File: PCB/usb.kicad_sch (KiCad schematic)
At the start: 53 parts, among them J2 Conn_ARM_SWD_TagConnect_TC2030, J4 TYPE-C-31-M-12, U10 FT2232HQ, U3 TPD2EUSB30, U4 TPD2EUSB30, U6 TPD2EUSB30, U8 TPS62132, U9 M93C56-WMN6TP, Y2 12MHz

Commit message: fixing a bunch of footprints to standardize
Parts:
- C124: footprint Capacitor_SMD:C_0402_1005Metric -> Capacitor_SMD:C_0603_1608Metric
- C92: footprint Capacitor_SMD:C_0402_1005Metric -> Capacitor_SMD:C_1206_3216Metric
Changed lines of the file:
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@@
 			)
 		)
-		(property "Footprint" "Capacitor_SMD:C_0402_1005Metric"
+		(property "Footprint" "Capacitor_SMD:C_0603_1608Metric"
 			(at 97.4852 38.1 0)
 			(effects
@@
 			)
 		)
-		(property "Footprint" "Capacitor_SMD:C_0402_1005Metric"
+		(property "Footprint" "Capacitor_SMD:C_1206_3216Metric"
 			(at 195.2752 48.26 0)
 			(effects

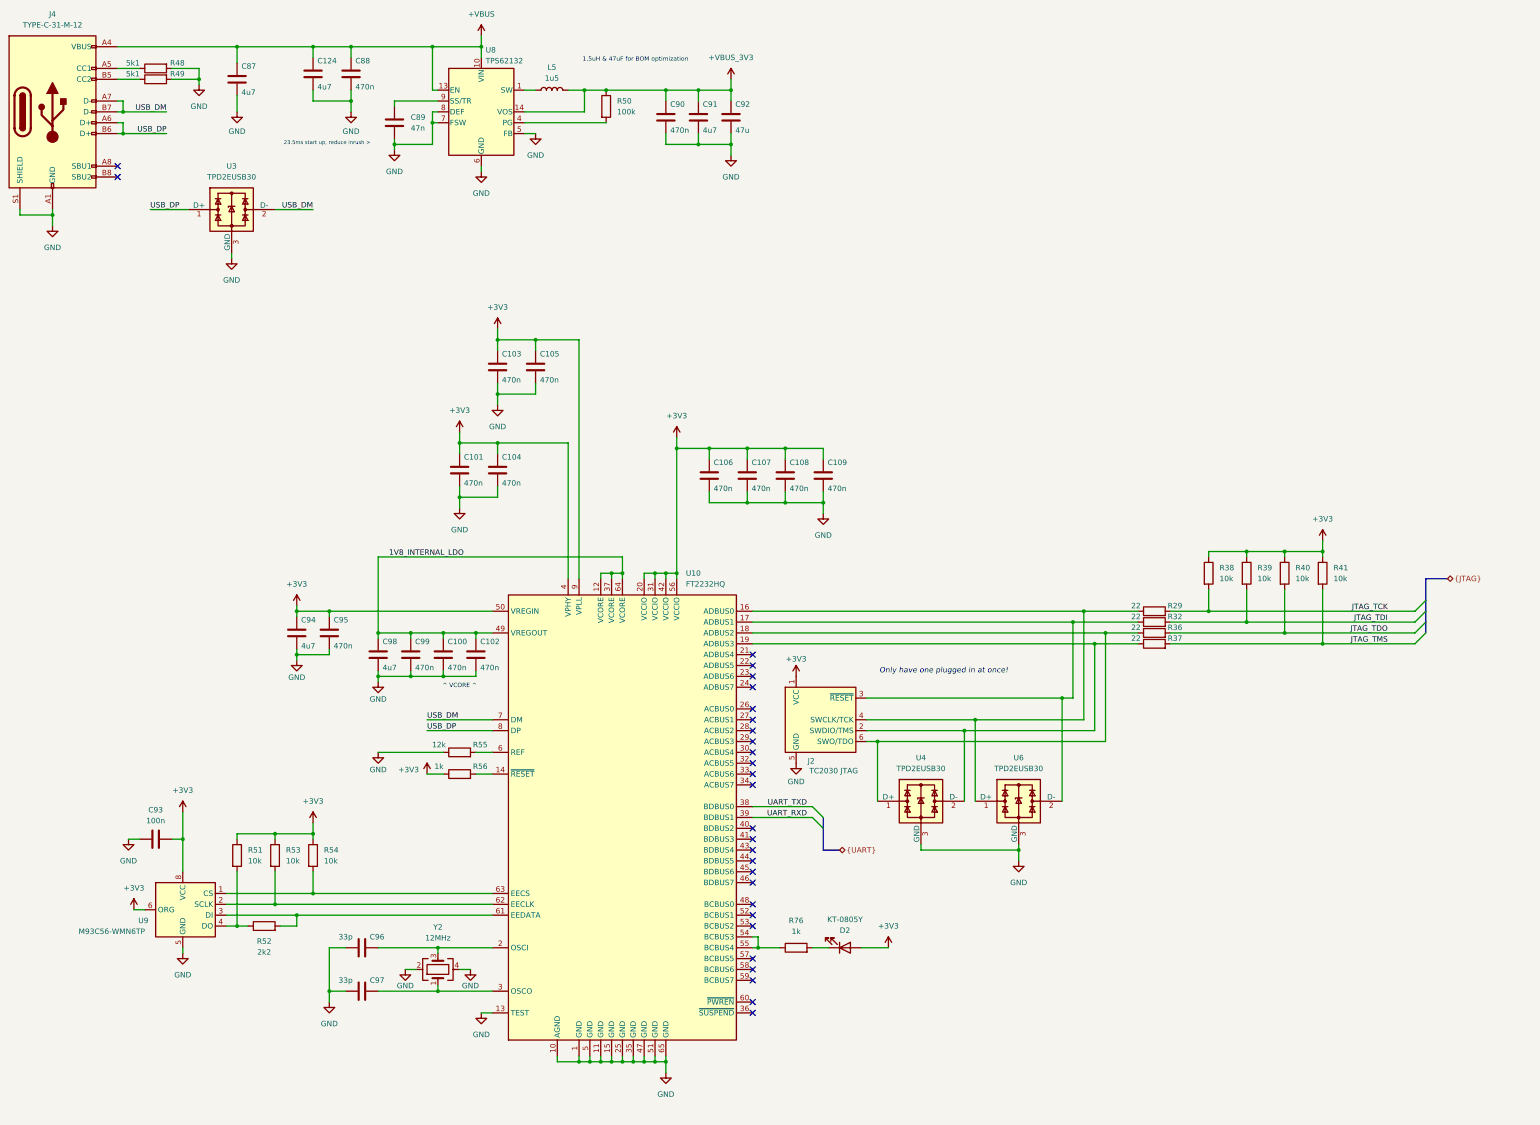
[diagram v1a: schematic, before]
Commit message: workingng on organizing the board
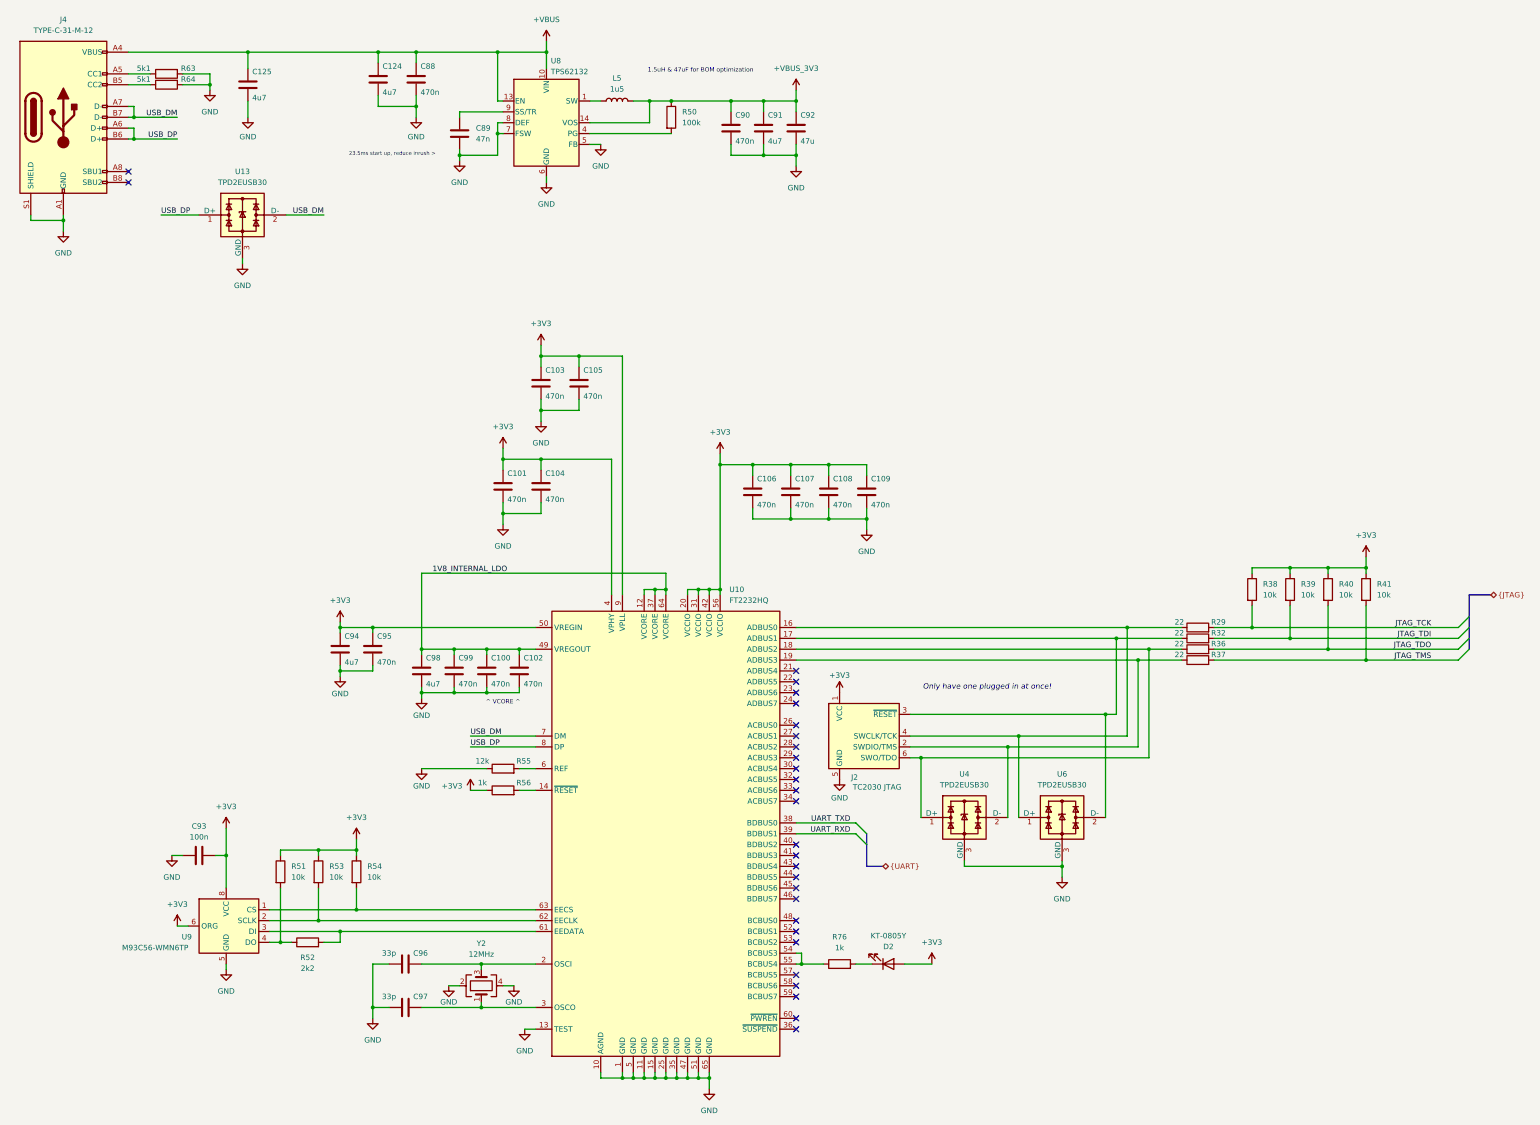
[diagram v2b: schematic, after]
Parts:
- removed C87: 4u7, Capacitor_SMD:C_0603_1608Metric, symbol Device:C
- removed R48, R49: 5k1, Resistor_SMD:R_0402_1005Metric, symbol Device:R
- removed U3: TPD2EUSB30, Package_TO_SOT_SMD:Texas_DRT-3, symbol Power_Protection:TPD2EUSB30
- added C125: 4u7, Capacitor_SMD:C_0603_1608Metric, symbol Device:C
- added R63, R64: 5k1, Resistor_SMD:R_0402_1005Metric, symbol Device:R
- added U13: TPD2EUSB30, Package_TO_SOT_SMD:Texas_DRT-3, symbol Power_Protection:TPD2EUSB30
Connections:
- net +VBUS: now also C125.1
- net GND: now also C125.2, R63.2, R64.2, U13.3 (GND)
- net USB_DM: now also U13.2 (D-)
- net USB_DP: now also U13.1 (D+)
- net at J4.B5 (CC2): now also R64.1
- net at J4.A5 (CC1): now also R63.1
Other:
- moved on the sheet: C100, C101, C102, C103, C104, C105, C106, C107, C108, C109, C124, C88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
